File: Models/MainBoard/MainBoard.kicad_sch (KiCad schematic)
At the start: 4 parts

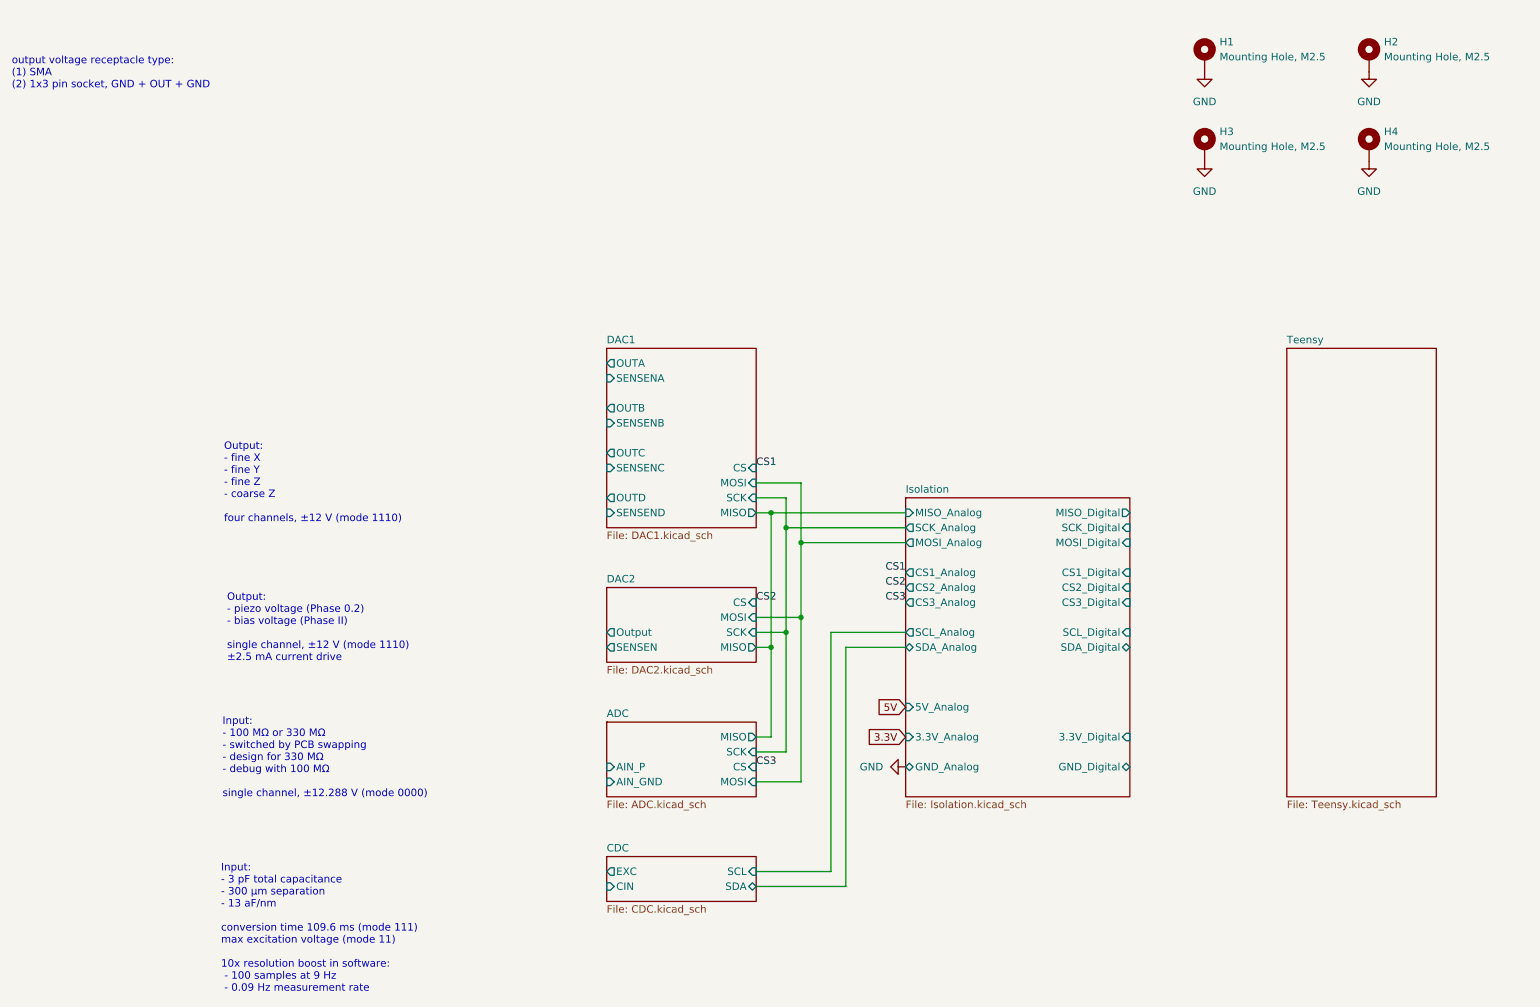
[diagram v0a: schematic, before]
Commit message: Save progress
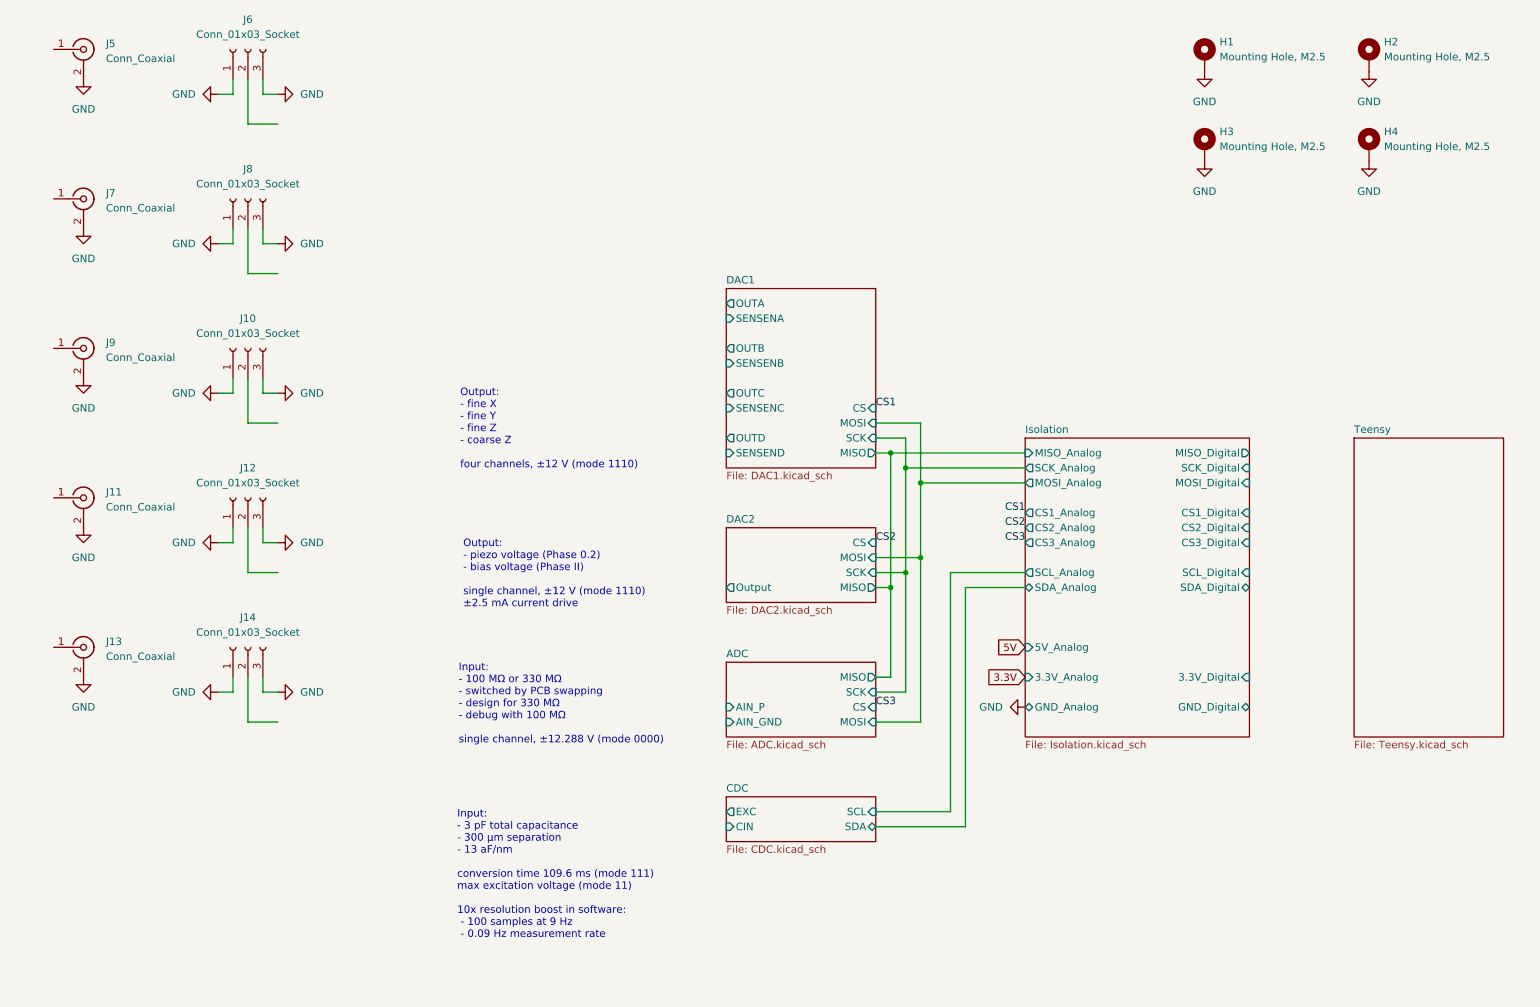
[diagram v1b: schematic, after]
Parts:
- added J10, J12, J14, J6, J8: Conn_01x03_Socket, symbol Connector:Conn_01x03_Socket
- added J11, J13, J5, J7, J9: Conn_Coaxial, symbol Connector:Conn_Coaxial
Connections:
- net GND: now also J10.1 (Pin_1), J10.3 (Pin_3), J11.2 (Ext), J12.1 (Pin_1), J12.3 (Pin_3), J13.2 (Ext), J14.1 (Pin_1), J14.3 (Pin_3), J5.2 (Ext), J6.1 (Pin_1), J6.3 (Pin_3), J7.2 (Ext), J8.1 (Pin_1), J8.3 (Pin_3), J9.2 (Ext)
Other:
- sheet DAC2 ports: added none; removed SENSEN
- note removed: "output voltage receptacle type: (1) SMA (2) 1x3 pin socket, GND + OUT + GND"
